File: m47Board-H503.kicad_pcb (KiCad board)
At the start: 4 copper layers, 40 x 34 mm, 44 parts, among them J1 USB_C_Receptacle_USB2.0_16P, J3 Conn_01x15_Pin, J4 Conn_01x10_Pin, J5 Conn_01x15_Pin, SW1 SW_Push, SW2 SW_Push, SW3 SW_Push, U1 AP2114H-3.3TRG1, U2 STM32H503CBTx, U3 USBLC6-2SC6, Y1 CX3225FB16000F0FZZH1 16MHz, Y2 ABS07-32.768KHZ-T

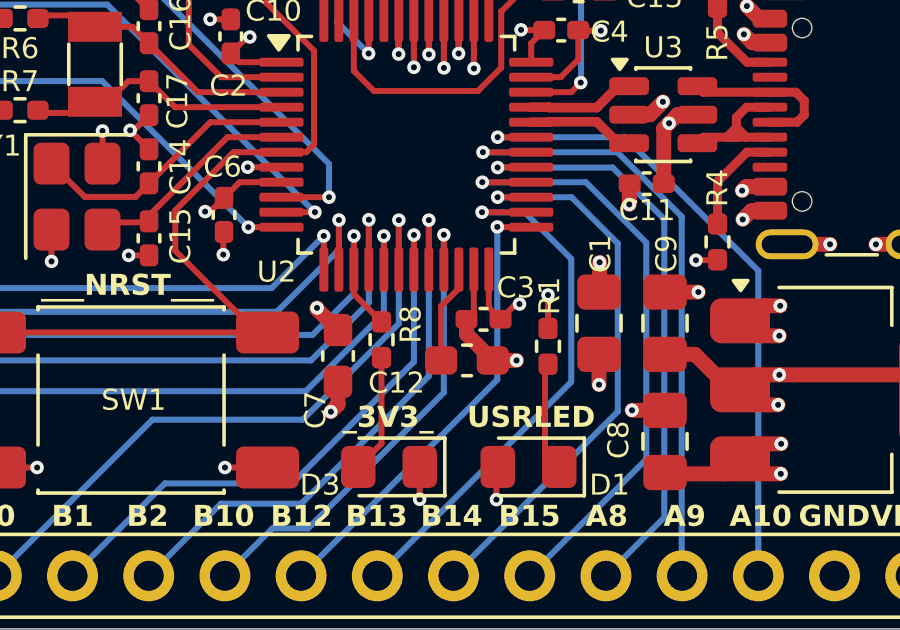
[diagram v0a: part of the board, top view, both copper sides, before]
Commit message: Clean DRC
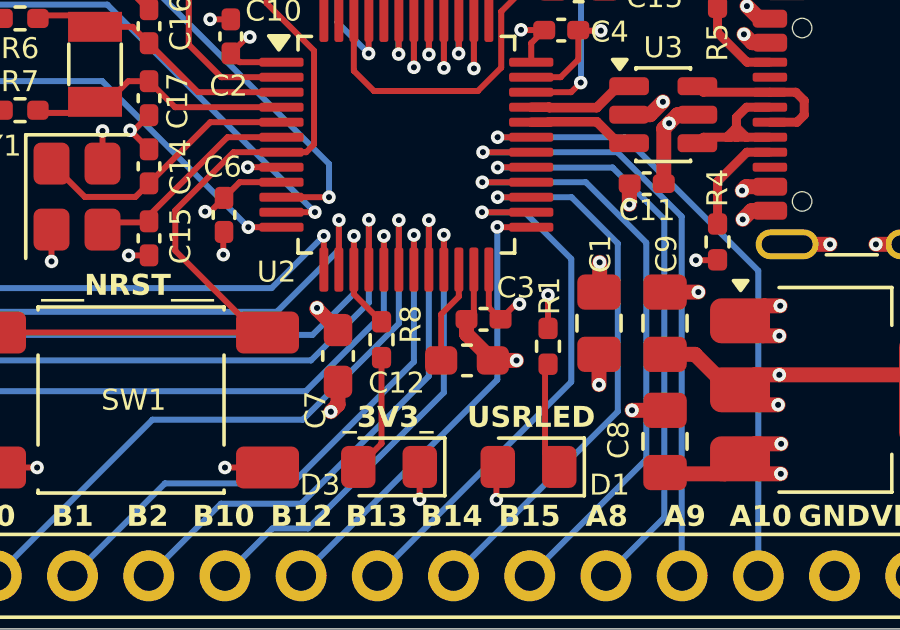
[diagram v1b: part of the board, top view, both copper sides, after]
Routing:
- net +3.3V: track 31.5 -> 33.7 mm
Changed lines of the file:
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@@
 	)
 	(gr_text "m47Board-H503"
-		(at 158.35 90.7 0)
+		(at 158.35 90.5 0)
 		(layer "B.SilkS" knockout)
 		(effects
@@
 	)
 	(segment
+		(start 121.78 118.23)
+		(end 121.78 118.22)
+		(width 0.5)
+		(layer "In2.Cu")
+		(net "+3.3V")
+	)
+	(segment
+		(start 121.78 118.22)
+		(end 123.3 116.7)
+		(width 0.5)
+		(layer "In2.Cu")
+		(net "+3.3V")
+	)
+	(segment
 		(start 151.885 101.11)
 		(end 150.9 100.125)
@@
 	)
 	(segment
-		(start 142.2775 108.650988)
-		(end 142.2775 108.0225)
+		(start 141.6875 111.05)
+		(end 141.6875 109.5125)
 		(width 0.2)
 		(layer "F.Cu")
@@
 	)
 	(segment
-		(start 141.6875 111.05)
-		(end 141.6875 109.240988)
+		(start 142.2775 108.9225)
+		(end 142.2775 108.0225)
 		(width 0.2)
 		(layer "F.Cu")
@@
 	)
 	(segment
-		(start 141.6875 109.240988)
-		(end 142.2775 108.650988)
+		(start 141.6875 109.5125)
+		(end 142.2775 108.9225)
 		(width 0.2)
 		(layer "F.Cu")
